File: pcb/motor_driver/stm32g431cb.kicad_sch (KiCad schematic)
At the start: 44 parts, among them J3 Conn_ARM_JTAG_SWD_10, J5 Conn, Q1 BSS138, SW1 SKRPACE010, SW2 SKRPACE010, U10 STM32G431CB, U12 MCP2562-E-SN, Y1 XRCGB16M000FXN02R0

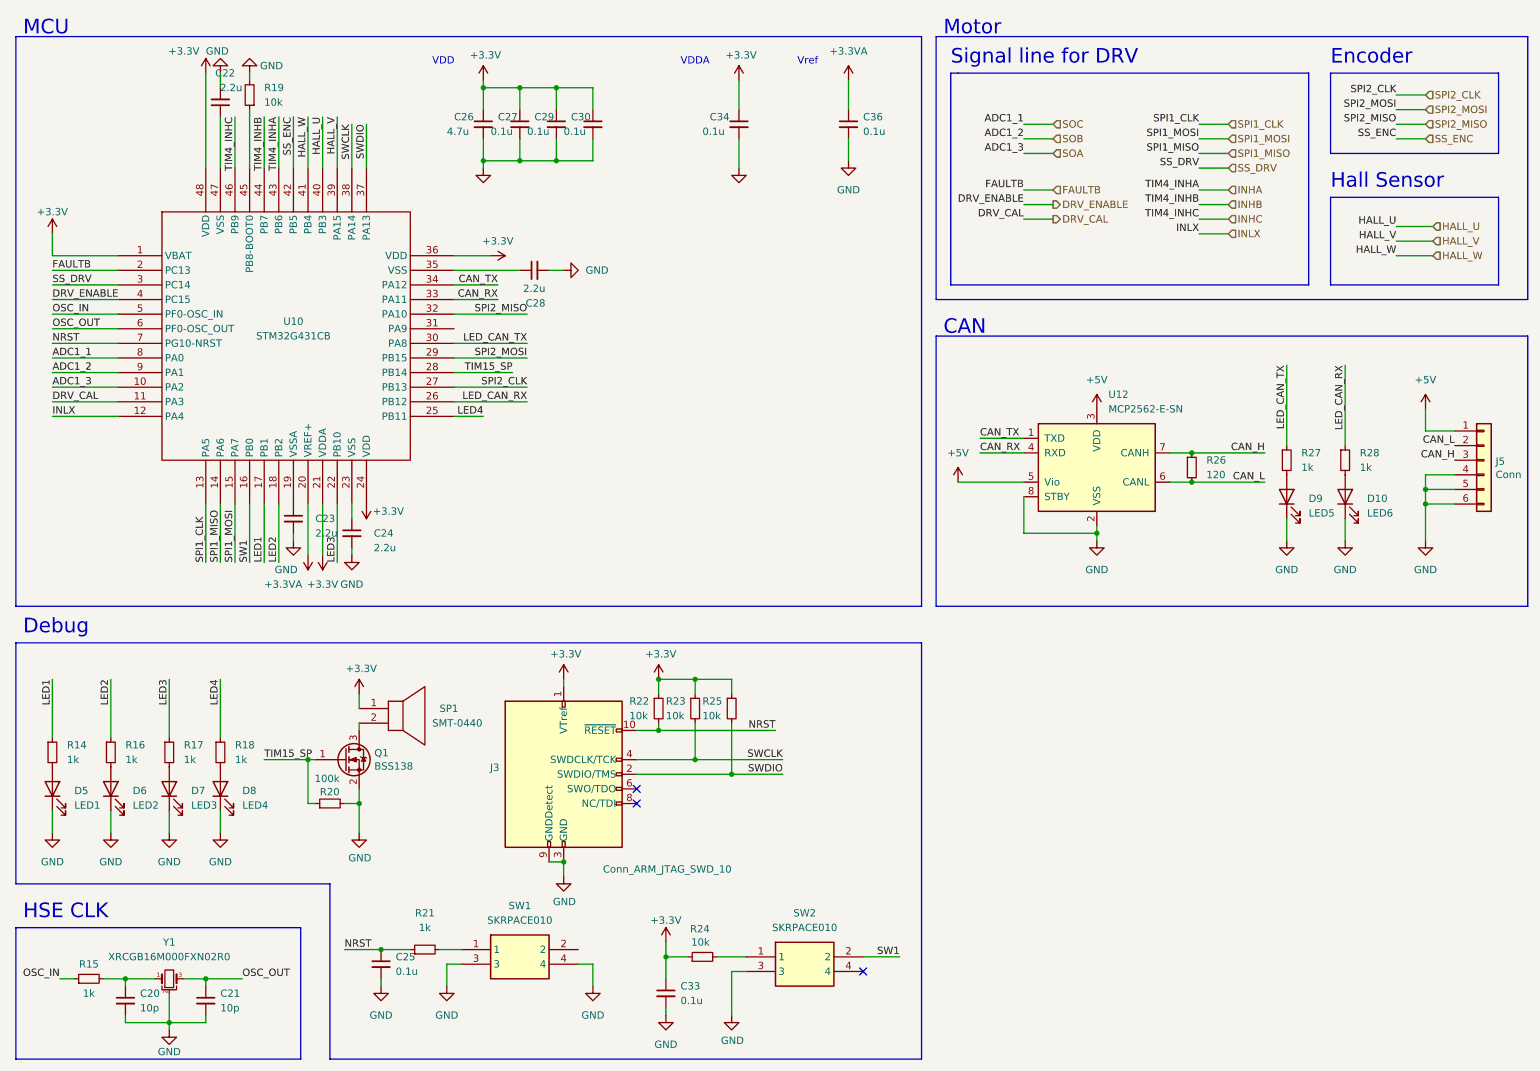
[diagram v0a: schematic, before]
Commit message: chore: commit before starting to develop v1.2
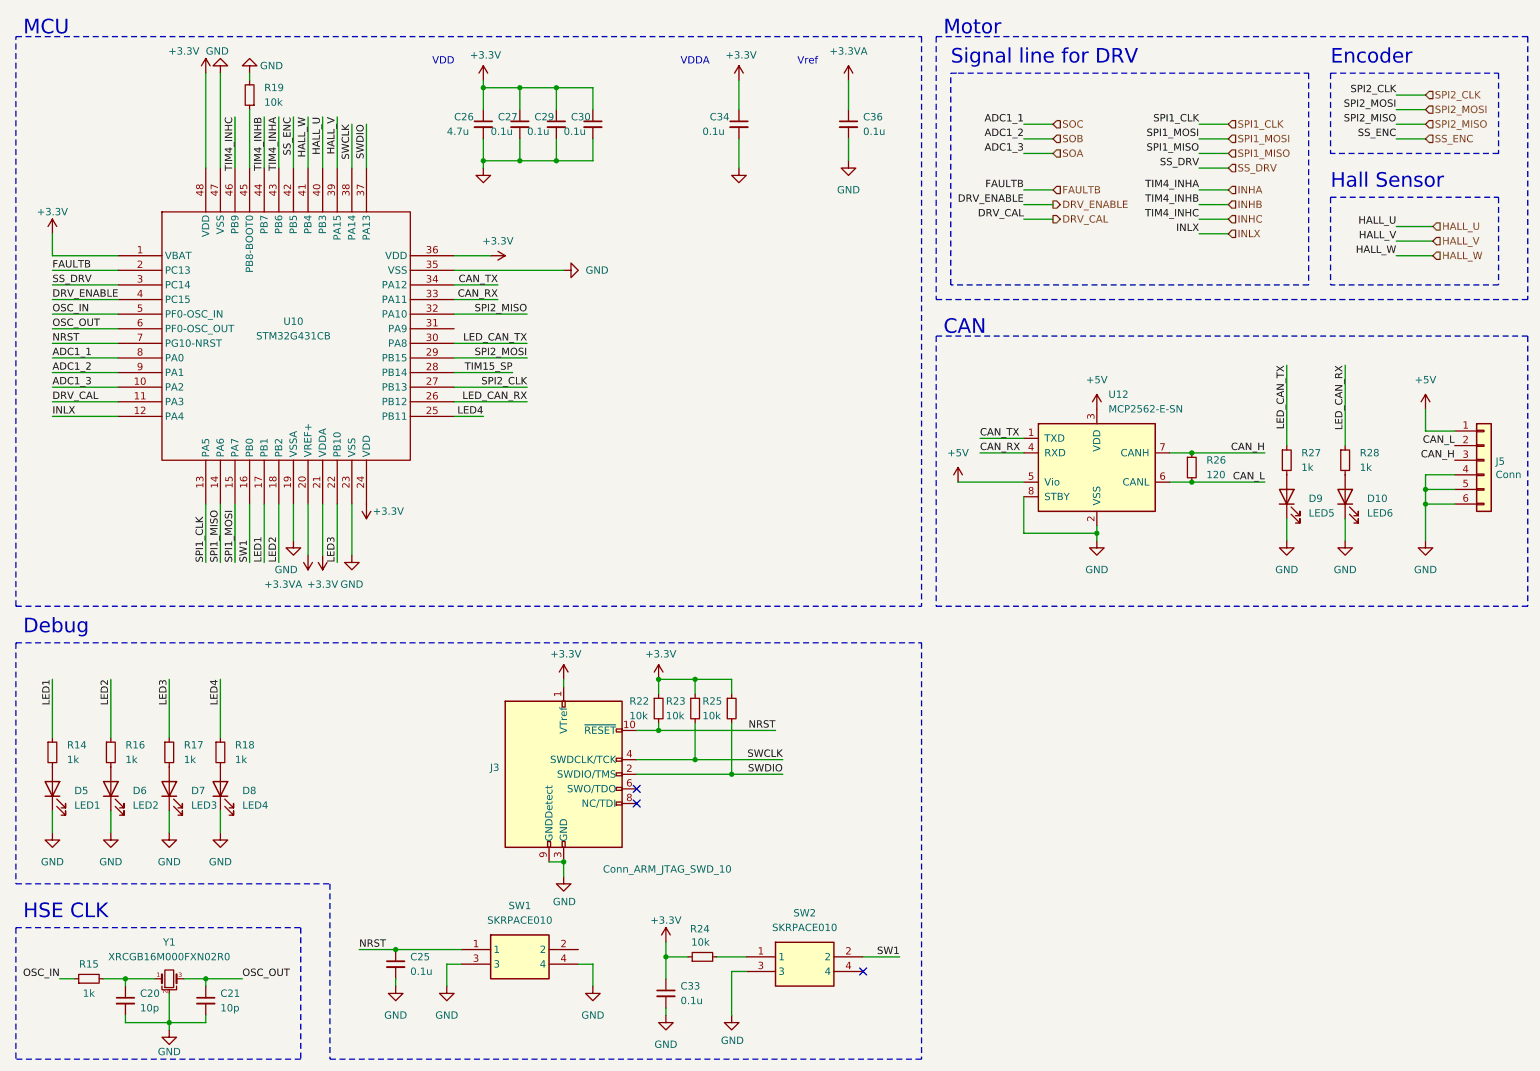
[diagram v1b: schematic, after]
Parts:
- removed C22, C23, C24, C28: 2.2u, Capacitor_SMD:C_0402_1005Metric, symbol Device:C_Small
- removed Q1: BSS138, Package_TO_SOT_SMD:SOT-23, symbol Transistor_FET:BSS138
- removed R20: 100k, Resistor_SMD:R_0201_0603Metric, symbol Device:R_Small
- removed R21: 1k, Resistor_SMD:R_0603_1608Metric_Pad0.98x0.95mm_HandSolder, symbol Device:R_Small
- removed SP1: SMT-0440, omni:STM0440-T-R, symbol My_Device:SMT-0440
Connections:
- net GND: now also U10.19 (VSSA), U10.23 (VSS), U10.35 (VSS), U10.47 (VSS)
- net NRST: now also SW1.1
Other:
- moved on the sheet: C25
